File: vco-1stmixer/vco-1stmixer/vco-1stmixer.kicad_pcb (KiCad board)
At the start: 2 copper layers, 91.7 x 48.8 mm, 48 parts, among them J101 VCO Control In, J102 1st IF Out, J103 VCO Sample, J104 RF In, J105 Conn_01x02, U101 POS-200, U102 MAV-11, U103 MAV-11, U104 TUF-1H+

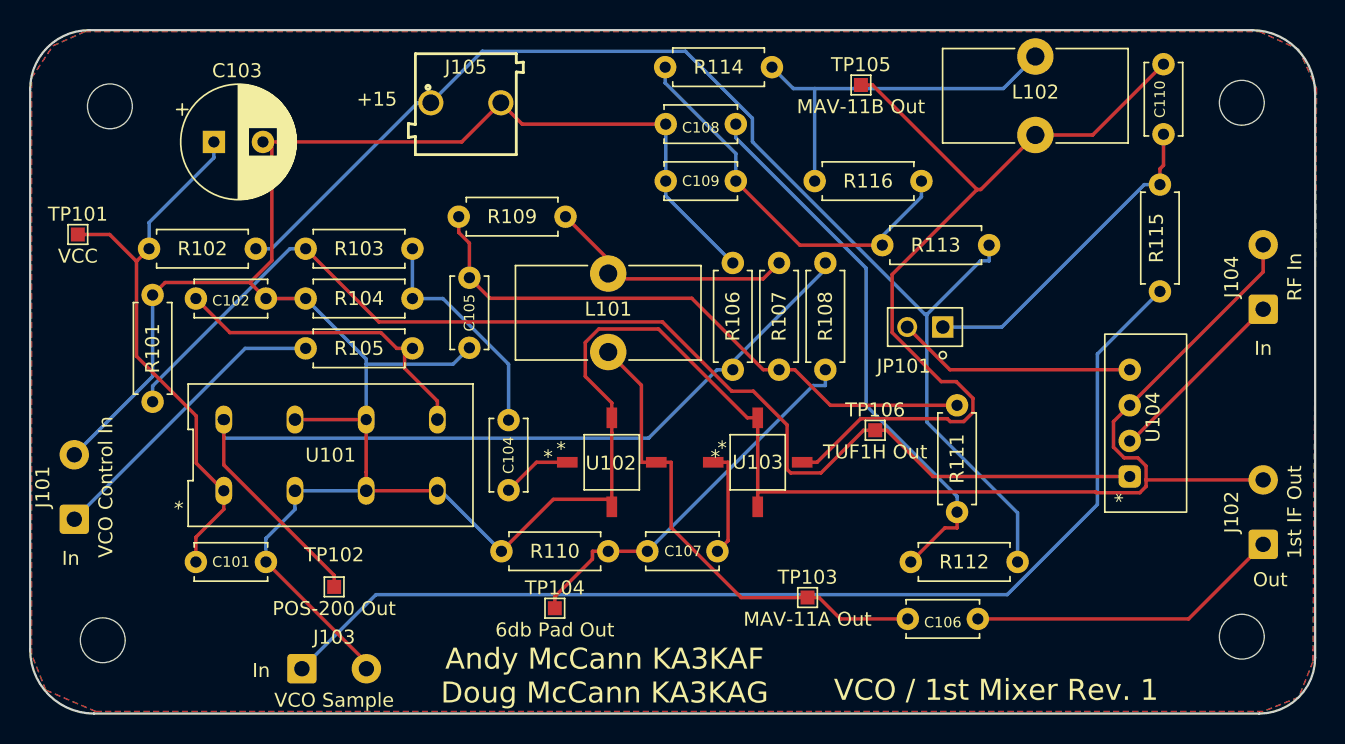
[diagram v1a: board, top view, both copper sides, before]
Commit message: 1st mixer VCO pcb rev 2
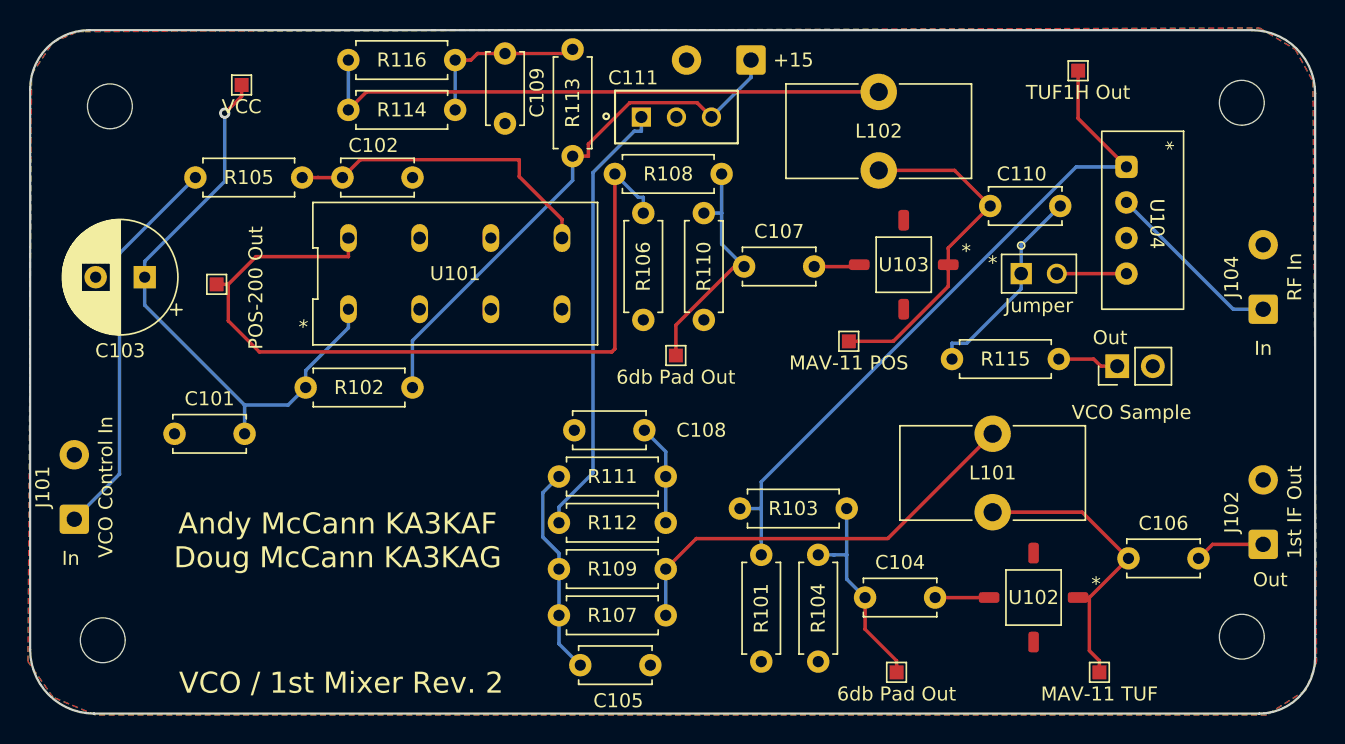
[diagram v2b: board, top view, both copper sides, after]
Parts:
- added C111: .001, spectrum-analyzer:DSS1N_MUR, F.Cu at (135.7, 84.8)
- added TP107: 6db Pad Out, TestPoint:TestPoint_Pad_1.0x1.0mm, F.Cu at (153.9, 124.4)
- J103: footprint Connector_Wire:SolderWire-0.5sqmm_1x02_P4.6mm_D0.9mm_OD2.1mm -> Connector_PinHeader_2.54mm:PinHeader_1x02_P2.54mm_Vertical
- J105: value Conn_01x02 -> +15; footprint vco-1stmixer:691103110002 -> Connector_Wire:SolderWire-0.5sqmm_1x02_P4.6mm_D0.9mm_OD2.1mm
- TP103: value MAV-11A Out -> MAV-11 TUF
- TP105: value MAV-11B Out -> MAV-11 POS
- moved J103 62.1 mm to (169.6, 102.6), turned to 90 degrees
- moved R101 50.7 mm to (144.2, 123.7), turned to 90 degrees
- moved R104 44.8 mm to (148.3, 123.7), turned to 90 degrees
- moved R103 36.1 mm to (142.7, 112.8)
- moved R116 34.4 mm to (114.8, 80.7)
- moved U102 31.6 mm to (163.7, 119.1)
- moved R114 30.4 mm to (114.8, 84.3), turned to 0 degrees
- moved L101 29.7 mm to (160.7, 107.4)
- moved TP106 29.5 mm to (166.8, 81.5)
- moved R111 28.9 mm to (129.8, 110.5), turned to 0 degrees
- moved C104 28.4 mm to (151.6, 119.1), turned to 0 degrees
- moved R107 26.4 mm to (137.4, 120.4), turned to 180 degrees
- moved R113 26.1 mm to (130.8, 80.0), turned to -90 degrees
- moved R109 26.1 mm to (137.4, 117.1)
- moved C105 26.1 mm to (136.3, 123.9), turned to 180 degrees
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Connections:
- J105 pad 1: Net-(J105-Pad1) -> /+15
- R102 pad 2: Net-(J105-Pad1) -> /+15
- R112 pad 2: Net-(J105-Pad1) -> Net-(C111-Pad1)
- R113 pad 2: Net-(J105-Pad1) -> /+15
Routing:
- net GND: track 243.1 -> 0.00 mm
- net Net-(J105-Pad1): track 90.0 -> 0.00 mm
- net Net-(J103-In): track 78.7 -> 4.38 mm
- net Net-(U103-RF_Out): track 63.6 -> 24.7 mm
- net /+15: track 0.00 -> 38.9 mm
- net Net-(U104-RF): track 86.0 -> 50.4 mm
- net Net-(C108-Pad2): track 39.7 -> 7.24 mm
- net Net-(C111-Pad1): track 0.00 -> 31.7 mm
- net Net-(C105-Pad2): track 43.2 -> 15.0 mm
- net Net-(J102-In): track 22.6 -> 5.03 mm
- net Net-(C109-Pad2): track 28.3 -> 12.3 mm
- net Net-(L102-Pad1): track 27.0 -> 41.9 mm
- net Net-(U102-RF_Out): track 35.2 -> 21.4 mm
- net Net-(L101-Pad1): track 18.1 -> 30.6 mm
- net Net-(JP101-J2): track 17.1 -> 4.97 mm
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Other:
- board text added: "VCO / 1st Mixer Rev. 2"
- board text removed: "+15"
- board text removed: "VCO / 1st Mixer Rev. 1"
